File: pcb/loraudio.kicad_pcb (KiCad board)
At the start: 2 copper layers, 70 x 50 mm, 14 parts

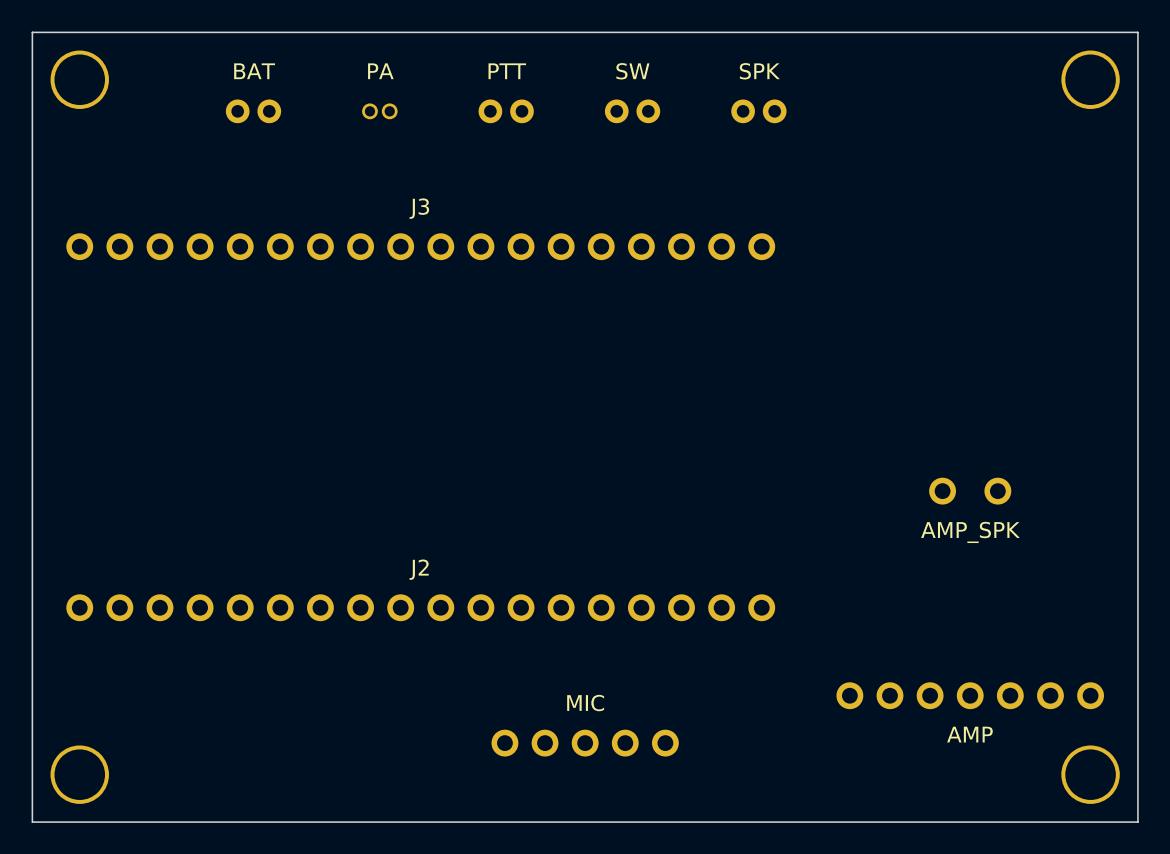
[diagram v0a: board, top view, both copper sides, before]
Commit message: ground plane
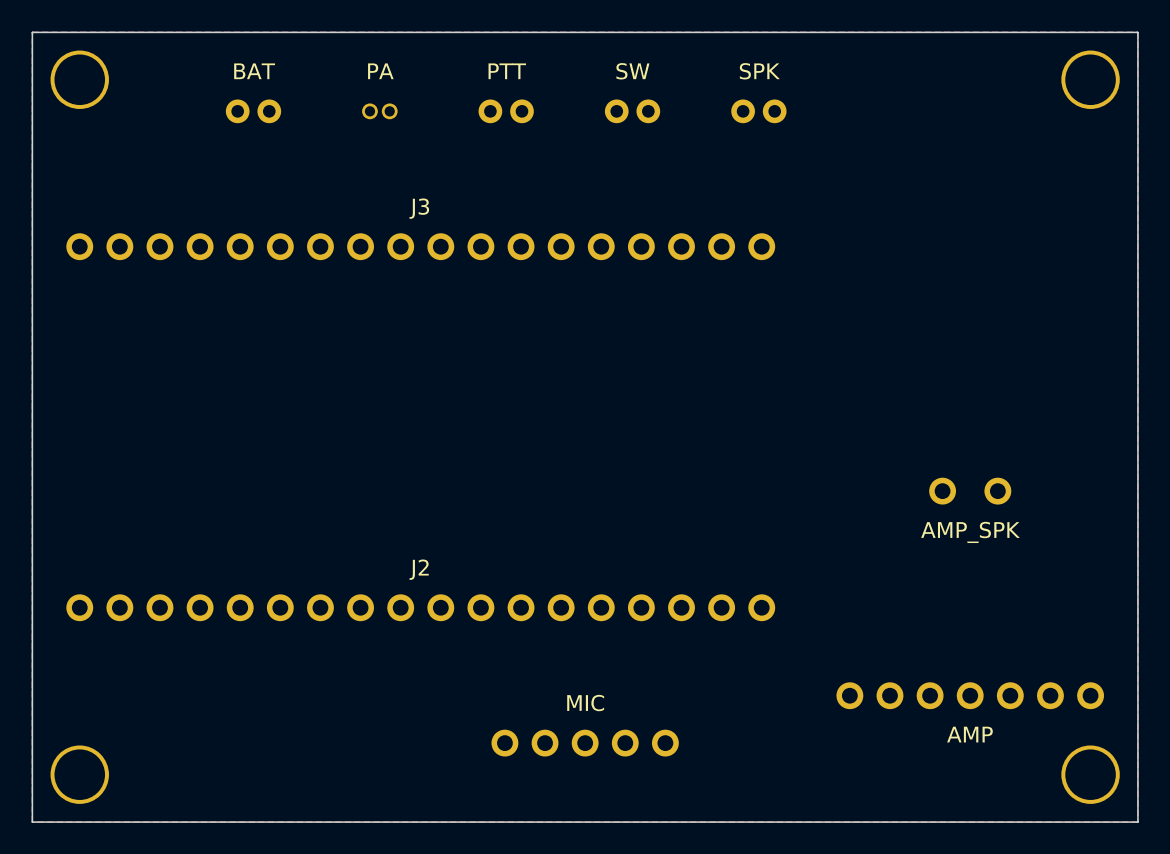
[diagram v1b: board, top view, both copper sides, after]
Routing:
- added copper zone on B.Cu, net GND
- added copper zone on F.Cu, net GND
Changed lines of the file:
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@@
+    )
+  )
+  (zone
+    (net 2)
+    (net_name "GND")
+    (layers "F.Cu" "B.Cu")
+    (hatch edge 0.5)
+    (connect_pads
+      (clearance 0.5)
+    )
+    (min_thickness 0.25)
+    (filled_areas_thickness no)
+    (fill yes
+      (thermal_gap 0.5)
+      (thermal_bridge_width 0.5)
+    )
+    (polygon
+      (pts
+        (xy 113 113) (xy 183 113) (xy 183 163) (xy 113 163)
+      )
     )
   )
